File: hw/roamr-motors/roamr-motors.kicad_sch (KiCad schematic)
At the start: 22 parts, among them J1 USB_C_Receptacle_USB2.0_14P, J10 JST_XH_S2B-XH-A-1, J2 USB_C_Receptacle_USB2.0_14P, J3 JST_XH_S2B-XH-A-1, J4 JST_XH_S2B-XH-A-1, J5 JST_PH_B3B-PH-SM4-TB, J6 JST_PH_B3B-PH-SM4-TB, J7 JST_SH_BM06B-SRSS-TB, J8 JST_SH_BM06B-SRSS-TB, J9 JST_XH_S2B-XH-A-1

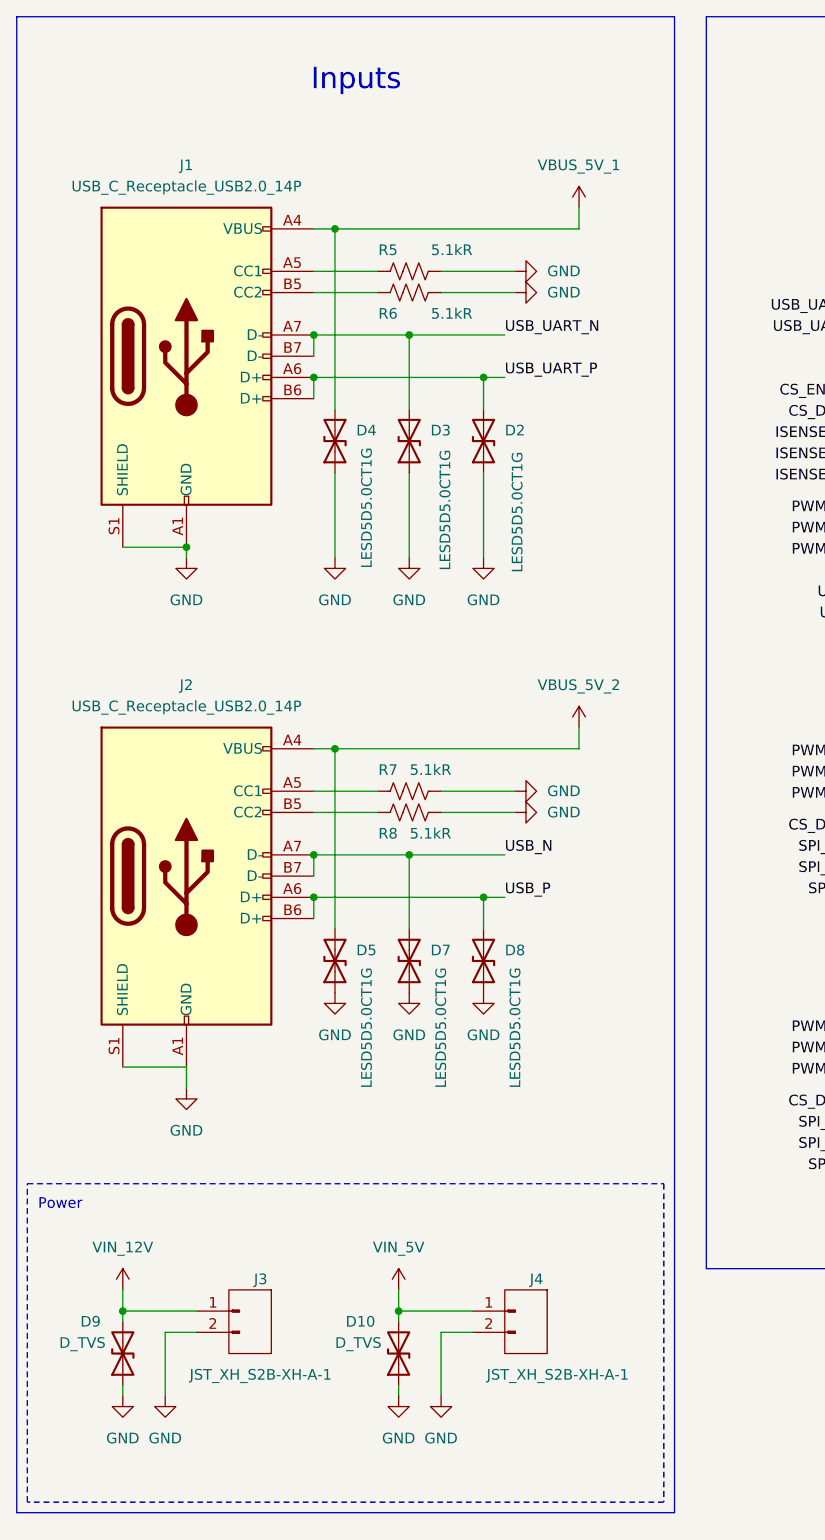
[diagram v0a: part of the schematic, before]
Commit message: some more layout
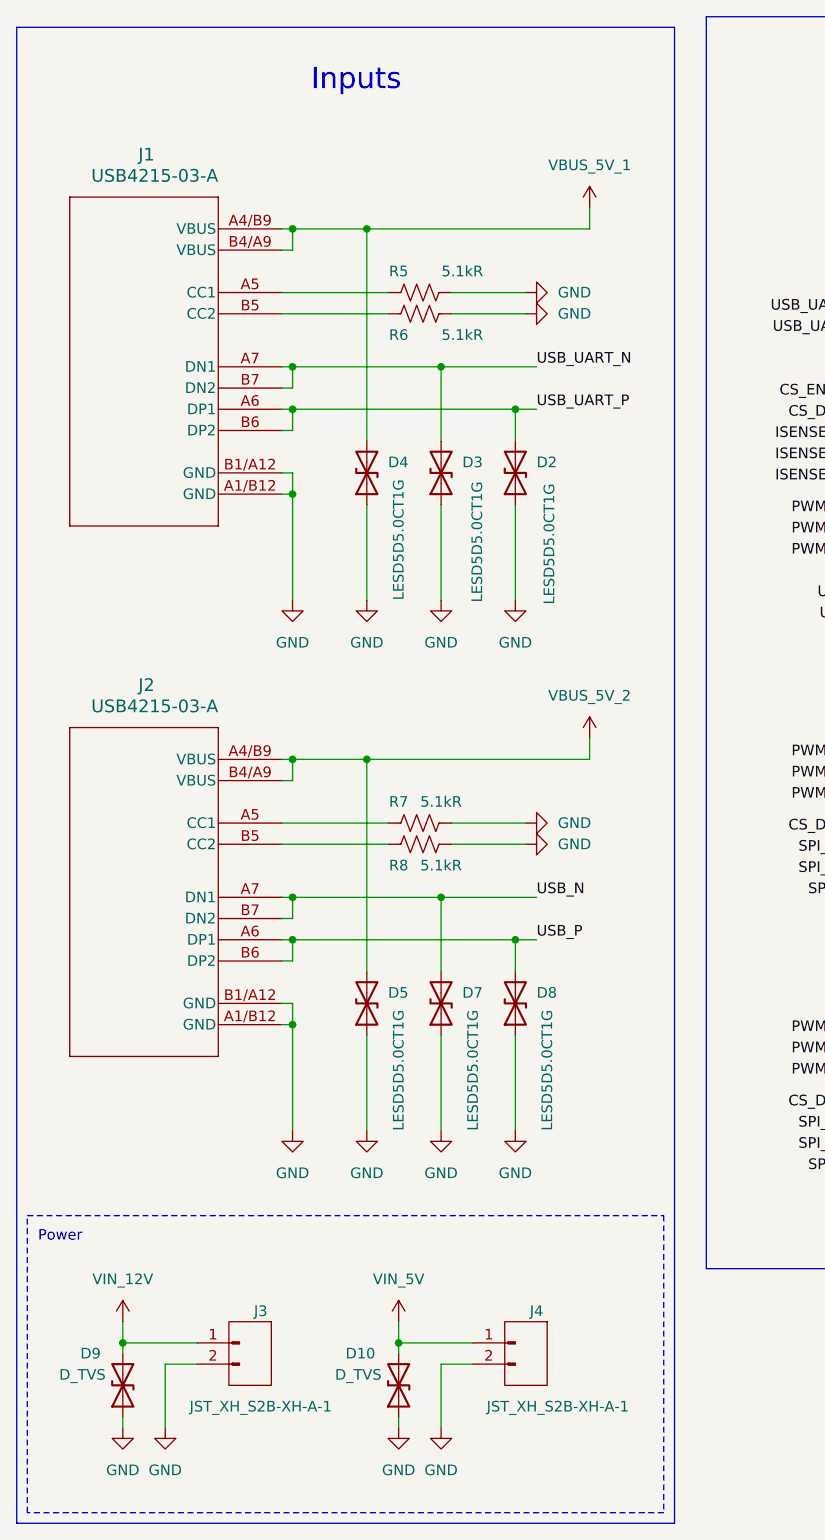
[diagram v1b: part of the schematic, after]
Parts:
- removed J1, J2: USB_C_Receptacle_USB2.0_14P, USB4215_03_A:CONN_8p94X6p5X3p16_12L_GCC, symbol Connector:USB_C_Receptacle_USB2.0_14P
- added J1, J2: USB4215-03-A, CONN_8p94X6p5X3p16_12L_GCC, symbol USB4215_03_A:USB4215-03-A
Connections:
- net GND: now also J1.A1/B12 (GND), J1.B1/A12 (GND), J2.A1/B12 (GND), J2.B1/A12 (GND)
- net USB_N: now also J2.A7 (DN1), J2.B7 (DN2)
- net USB_P: now also J2.A6 (DP1), J2.B6 (DP2)
- net USB_UART_N: now also J1.A7 (DN1), J1.B7 (DN2)
- net USB_UART_P: now also J1.A6 (DP1), J1.B6 (DP2)
- net VBUS_5V_1: now also J1.A4/B9 (VBUS), J1.B4/A9 (VBUS)
- net VBUS_5V_2: now also J2.A4/B9 (VBUS), J2.B4/A9 (VBUS)
- net at R5.1: now also J1.A5 (CC1)
- net at R8.1: now also J2.B5 (CC2)
- net at R7.1: now also J2.A5 (CC1)
- net at R6.1: now also J1.B5 (CC2)
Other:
- moved on the sheet: D10, D2, D3, D4, D5, D7, D8, D9, J3, J4, R5, R6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
